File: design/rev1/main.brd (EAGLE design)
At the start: 78 x 50 mm, 43 parts, among them J1 ICSP-HEADER1X6-0.1-ICSP-PADS, J2 HEADER-141X14-0.1-PADS, SW1 JS102000SAQN, SW2 JS102000SAQN, SW3 B3U-3000P, U1 PIC18F2XK20, U2 LIS3DSH, U3 APDS-9008

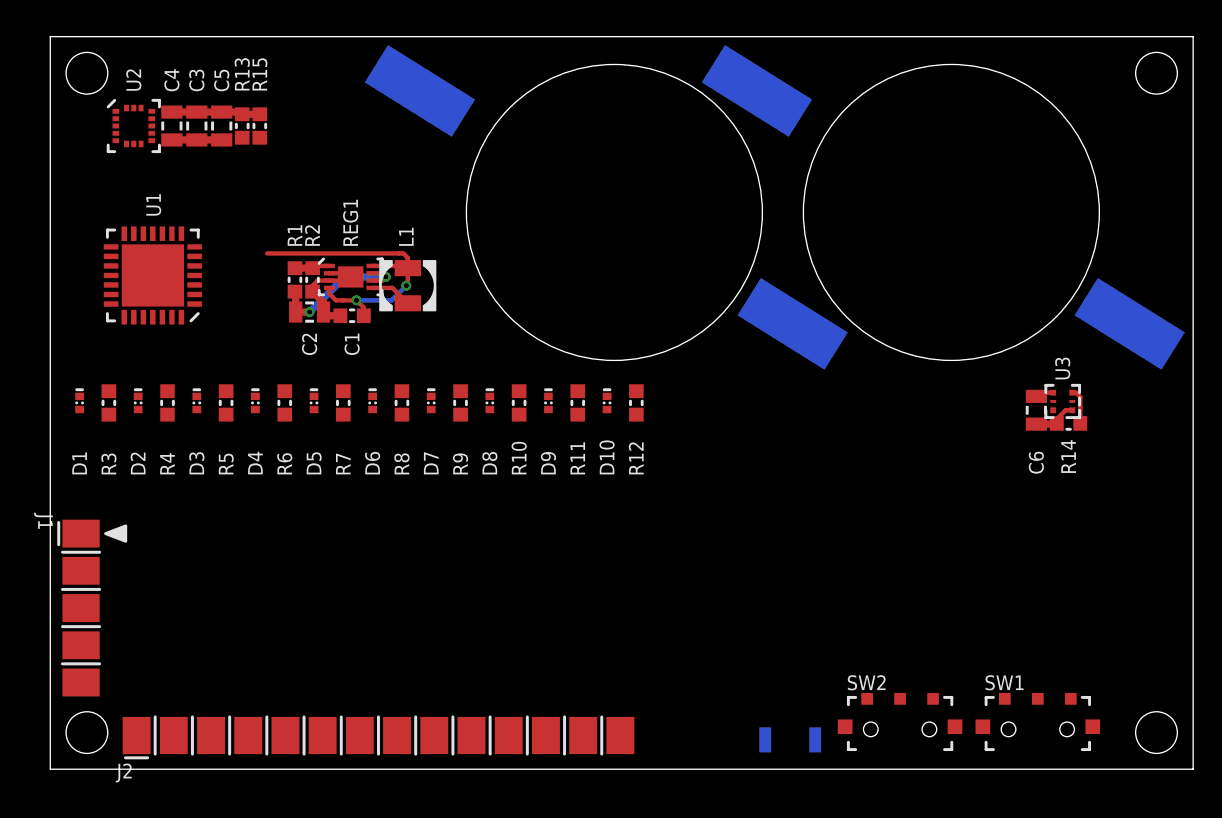
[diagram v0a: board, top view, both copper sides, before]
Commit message: [CNG] - more schematic and layout progress on rev1
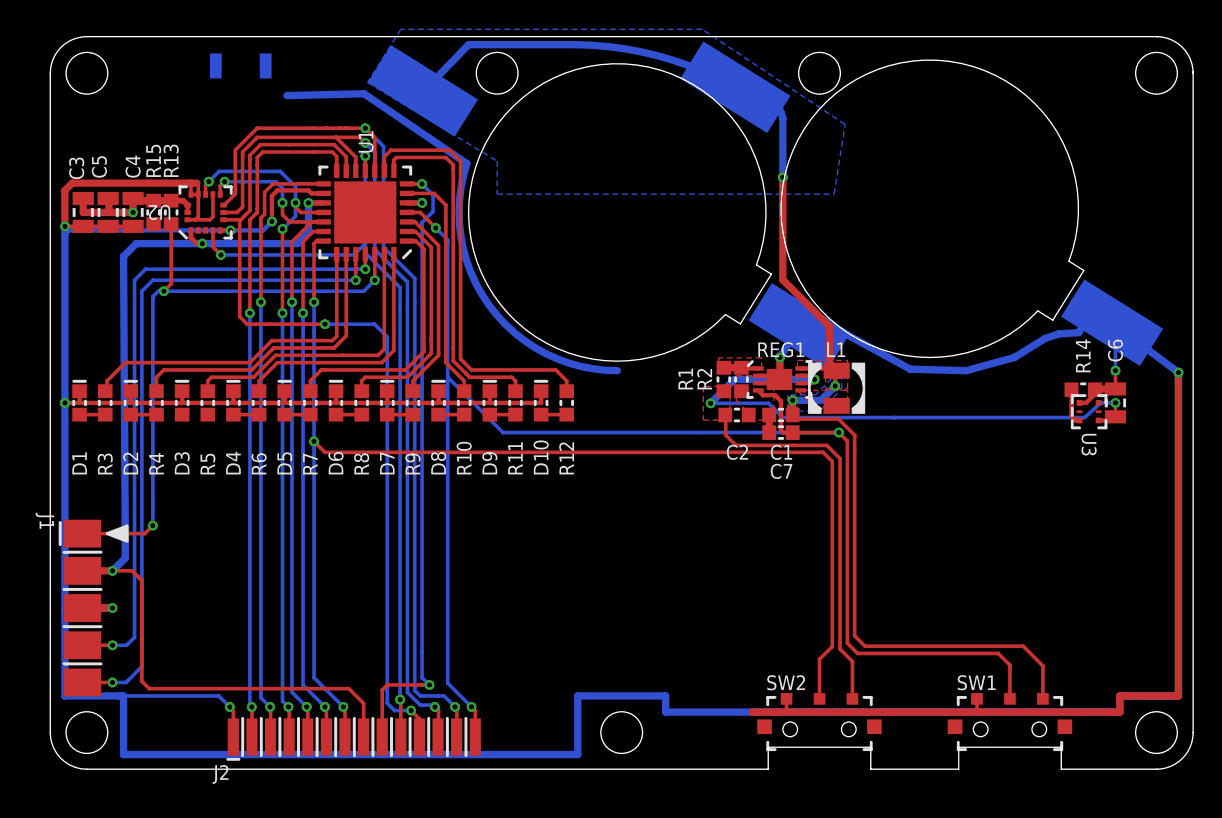
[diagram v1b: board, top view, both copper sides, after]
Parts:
- added C7: 0.1uF, matt:SMD-0603
- C2: device matt:SMD-0805 -> matt:SMD-0603
- D1, D10, D2, D3, D4, D5, D6, D7, D8, D9: value LED0402 -> LED0603; device matt:SMD-0402-P -> matt:SMD-0603-P
- J2: value HEADER-141X14-0.1-PADS -> HEADER-141X14-0.05-PADS; device matt:1X14-0.1-PADS -> matt:1X14-0.05-PADS
- moved SW3 59.3 mm to (13.0, 48.0), turned to 0 degrees
- moved L1 30.1 mm to (53.7, 26.0)
- moved REG1 30.1 mm to (49.8, 26.6)
- moved R2 30.0 mm to (47.2, 26.6)
- moved R1 30.0 mm to (46.0, 26.6)
- moved C1 30.0 mm to (49.9, 24.2)
- moved C2 30.0 mm to (46.9, 24.2)
- moved U1 15.1 mm to (21.5, 38.0)
- moved C3 11.1 mm to (2.25, 38.0)
- moved R15 9.35 mm to (7.05, 38.0)
- moved C5 8.45 mm to (3.95, 38.0)
- moved U2 7.67 mm to (10.6, 38.0), turned to 90 degrees
- moved R13 7.64 mm to (8.25, 38.0)
- moved C4 6.47 mm to (5.65, 38.0)
- moved SW2 5.50 mm to (52.5, 2.90)
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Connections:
- removed net N$1: B1.P$+, B2.P$+, SW1.SW$3
- new net V_BATT: B1.P$+, B2.P$+, C1.1, L1.P$1, REG1.8, SW1.SW$3
- net +3V3: now also J1.P$2
- net ACCEL_INT1: now also J2.P$4; no longer J2.P$11
- net ACCEL_INT2: now also J2.P$5; no longer J2.P$12
- net GND: now also C7.2, J2.P$1, SW1.SW$1; no longer J2.P$14
- net LIGHT_VSENSE: now also J2.P$6; no longer J2.P$10
- net PIC_CS: now also J2.P$13; no longer J2.P$4
- net PIC_EXT_FUNC: now also J2.P$9; no longer J2.P$13
- net PIC_RX: now also J2.P$3; no longer J2.P$2
- net PIC_SCK: now also J2.P$10; no longer J2.P$5
- net PIC_SDI: now also J2.P$12; no longer J2.P$7
- net PIC_SDO: now also J2.P$11; no longer J2.P$6
- net PIC_TX: now also J2.P$2; no longer J2.P$3
- net PROG_EN: now also J2.P$7; no longer J2.P$9
- net V_SW: now also C7.1, J2.P$14; no longer C1.1, J1.P$2, J2.P$1, L1.P$1, REG1.8
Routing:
- net GND: track 14.2 -> 342.9 mm, vias 0 -> 10
- net +3V3: track 18.1 -> 178.9 mm, vias 2 -> 7
- net V_BATT: track 0.00 -> 88.6 mm, vias 0 -> 3
- net PROG_EN: track 0.00 -> 87.8 mm, vias 0 -> 3
- net V_SW: track 21.7 -> 103.0 mm, vias 2 -> 3
- net PIC_CS: track 0.00 -> 62.1 mm, vias 0 -> 2
- net PIC_SDO: track 0.00 -> 60.2 mm, vias 0 -> 2
- net PIC_SDI: track 0.00 -> 60.1 mm, vias 0 -> 2
- net PIC_SCK: track 0.00 -> 53.9 mm, vias 0 -> 3
- net ACCEL_INT1: track 0.00 -> 48.1 mm, vias 0 -> 5
- net ACCEL_INT2: track 0.00 -> 46.9 mm, vias 0 -> 4
- net ICSP_CLK: track 0.00 -> 46.8 mm, vias 0 -> 2
- net PIC_TX: track 0.00 -> 46.5 mm, vias 0 -> 2
- net ICSP_DAT: track 0.00 -> 45.2 mm, vias 0 -> 2
- net ICSP_!MCLR!: track 0.00 -> 42.8 mm, vias 0 -> 3
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- added copper zone on layer 1, net +3V3
- added copper zone on layer 1, net GND
- added copper zone on layer 1, net N$3
- added copper zone on layer 1, net N$5
- added copper zone on layer 1, net V_BATT
- added copper zone on layer 16, net V_BATT
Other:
- outline, holes or cut-outs redrawn
